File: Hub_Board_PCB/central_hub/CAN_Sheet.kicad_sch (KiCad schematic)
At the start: 14 parts, among them J1 CAN_OUT, U3 MCP2515-xST, U4 TJA1050, Y2 20M

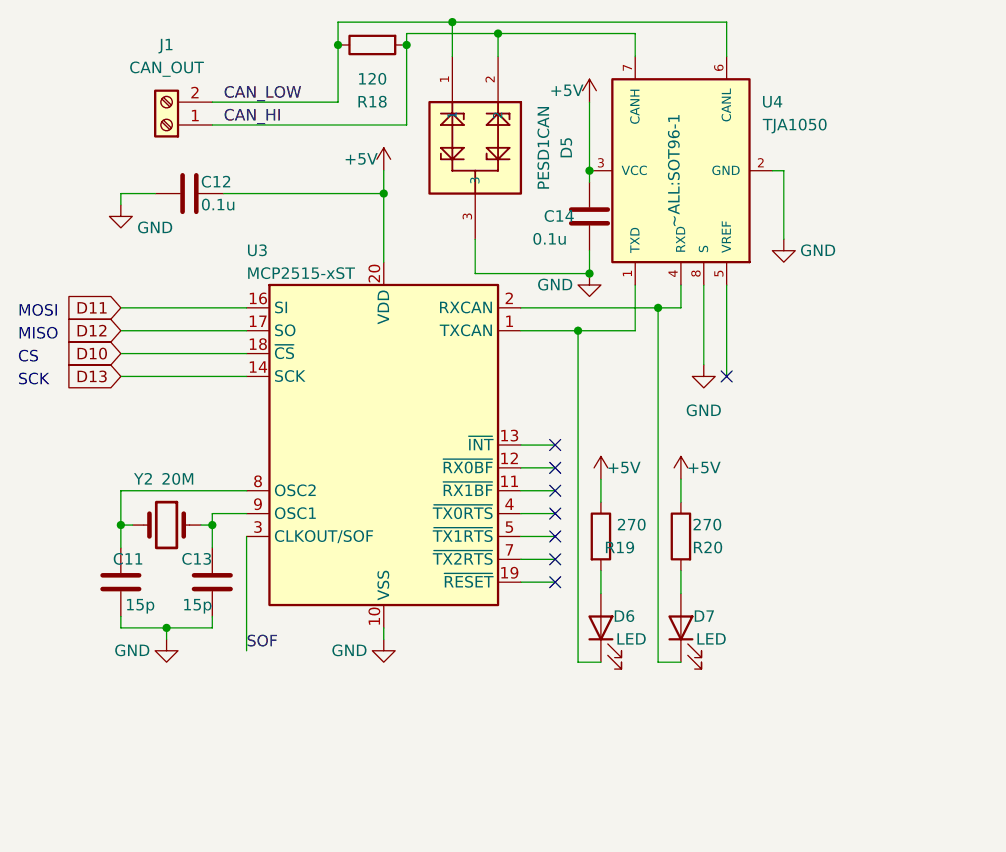
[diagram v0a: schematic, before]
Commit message: Schematic changes before sending to kim
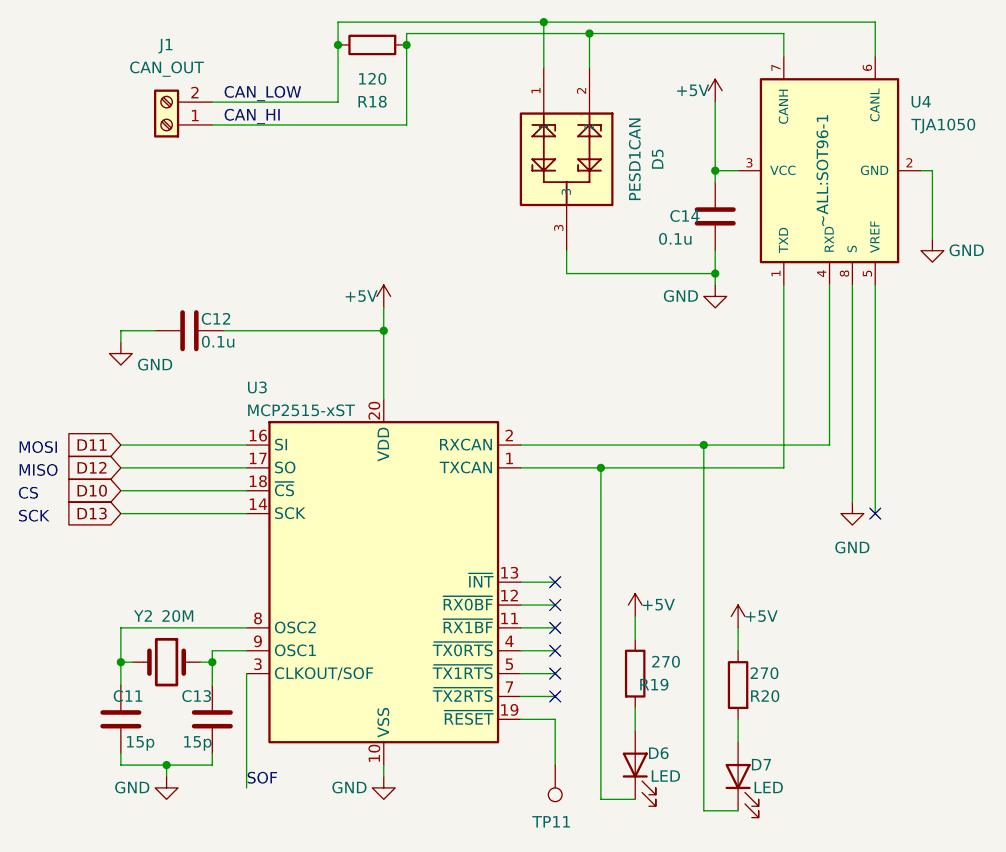
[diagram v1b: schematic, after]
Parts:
- added TP11: TestPoint, TestPoint:TestPoint_Pad_D1.0mm, symbol Connector:TestPoint
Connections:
- net at U3.19 (~{RESET}): now also TP11.1
- no-connect marks 8 -> 7
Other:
- moved on the sheet: C11, C12, C13, C14, D5, D6, D7, R19, R20, U3, U4, Y2

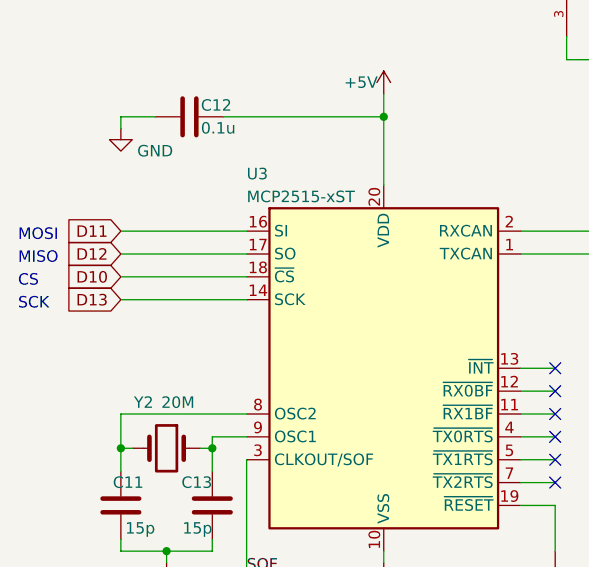
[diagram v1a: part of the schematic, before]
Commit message: Meeting layout updates
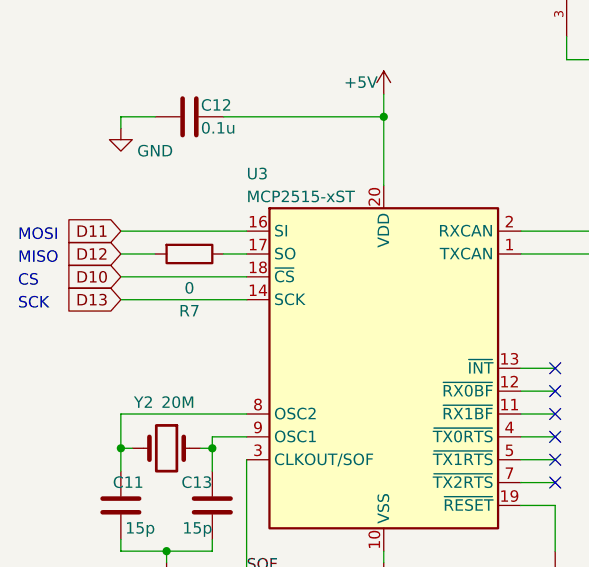
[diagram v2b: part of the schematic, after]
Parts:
- added R7: 0, Resistor_SMD:R_0402_1005Metric, symbol Device:R
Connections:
- net D12: now also R7.2; no longer U3.17 (SO)
- new net: R7.1, U3.17 (SO)
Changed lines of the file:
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@@
   (no_connect (at 76.2 87.63))
   (no_connect (at 76.2 82.55))
+  (wire (pts (xy 27.94 69.85) (xy 31.75 69.85))
+    (stroke (width 0) (type default))
+  )
   (wire (pts (xy 27.94 54.61) (xy 27.94 55.88))
     (stroke (width 0) (type default))
@@
     (stroke (width 0) (type default))
   )
+  (wire (pts (xy 39.37 69.85) (xy 41.91 69.85))
+    (stroke (width 0) (type default))
+  )
   (wire (pts (xy 92.71 67.31) (xy 92.71 107.95))
     (stroke (width 0) (type default))
@@
   )
   (wire (pts (xy 93.98 45.72) (xy 93.98 48.26))
-    (stroke (width 0) (type default))
-  )
-  (wire (pts (xy 27.94 69.85) (xy 41.91 69.85))
     (stroke (width 0) (type default))
   )
@@
         )
       )
+    )
+  )
+  (symbol (lib_id "Device:R") (at 35.56 69.85 270) (unit 1)
+    (in_bom yes) (on_board yes) (dnp no)
+    (property "Reference" "R7" (at 35.56 76.2 90)
+      (effects (font (size 1.27 1.27)))
+    )
+    (property "Value" "0" (at 35.56 73.66 90)
+      (effects (font (size 1.27 1.27)))
+    )
+    (property "Footprint" "Resistor_SMD:R_0402_1005Metric" (at 35.56 68.072 90)
+      (effects (font (size 1.27 1.27)) hide)
+    )
+    (property "Datasheet" "~" (at 35.56 69.85 0)
+      (effects (font (size 1.27 1.27)) hide)
+    )
+    (pin "1")
+    (pin "2")
+    (instances
+      (project "central_hub"
+        (path "/0d9ec66e-0fbf-4d12-9b83-adf78971a00b/a9a7affa-d8a7-4dcd-8fe3-0de6a2b29bd6"
+          (reference "R7") (unit 1)
+        )
+      )
+      (project "motor_board_pcb"
+        (path "/4ad82a24-c992-45c9-b523-12e12bcd6ced"
+          (reference "R?") (unit 1)
+        )
+        (path "/4ad82a24-c992-45c9-b523-12e12bcd6ced/63c66207-e5d4-4f6f-af8f-451675dc3930"
+          (reference "R16") (unit 1)
+        )
+      )
